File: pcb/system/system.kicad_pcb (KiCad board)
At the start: 2 copper layers, 136.7 x 117.6 mm, 33 parts, among them J1 Raspberry_Pi_4_GPIO, J2 Screw_Terminal_01x02, J3 Servo_1_Header, J4 Servo_2_Header, J5 Screw_Terminal_01x02, J6 Screw_Terminal_01x02, J7 Screw_Terminal_01x02, Q1 BS107A, Q2 BS107A, Q3 BS107A, Q4 BS107A, Q5 IRF520, Q6 IRF520, SW1 SW_SPST, SW2 SW_Push, U1 Teensy4.0

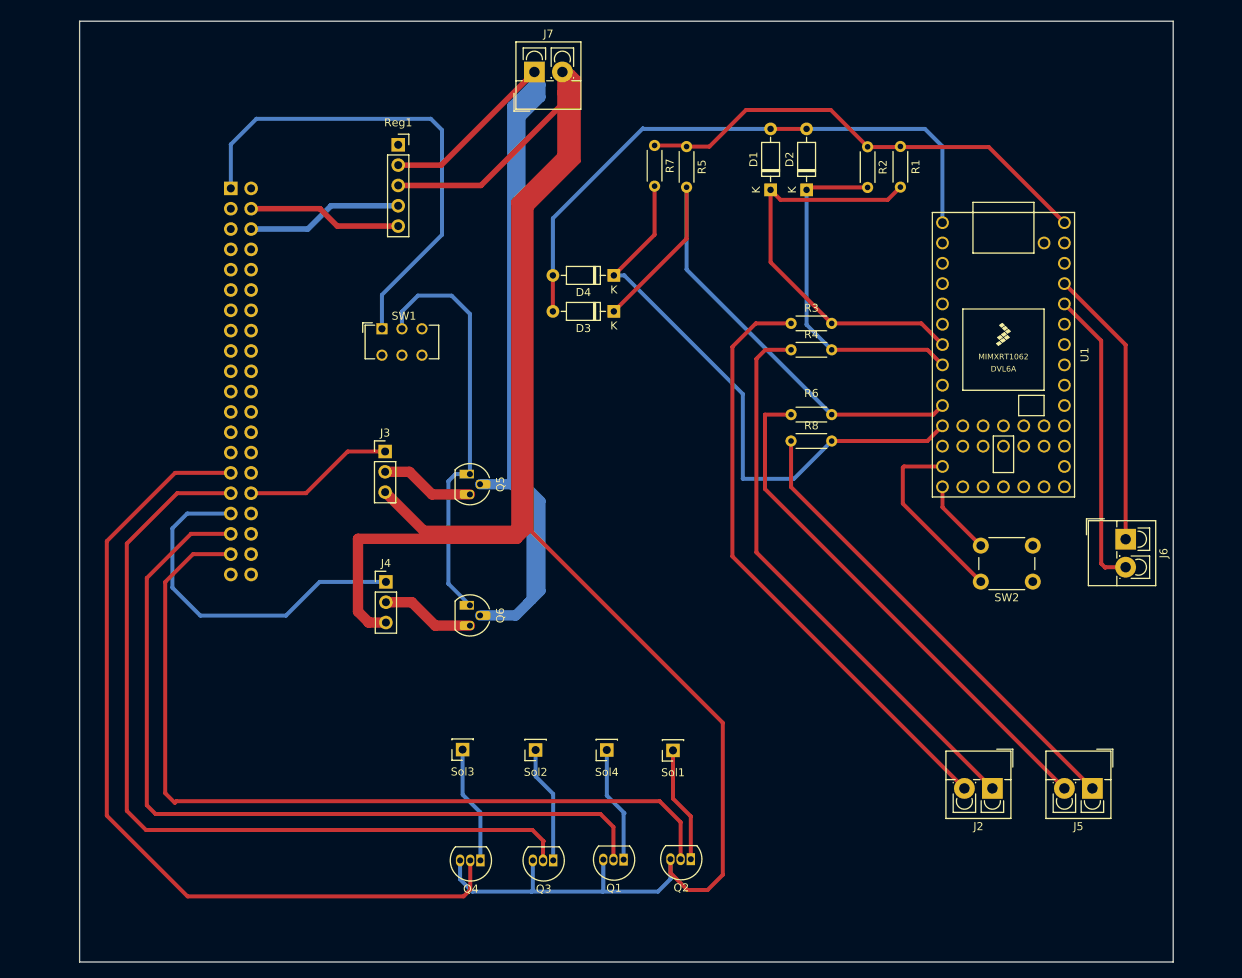
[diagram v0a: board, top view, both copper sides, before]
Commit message: awe
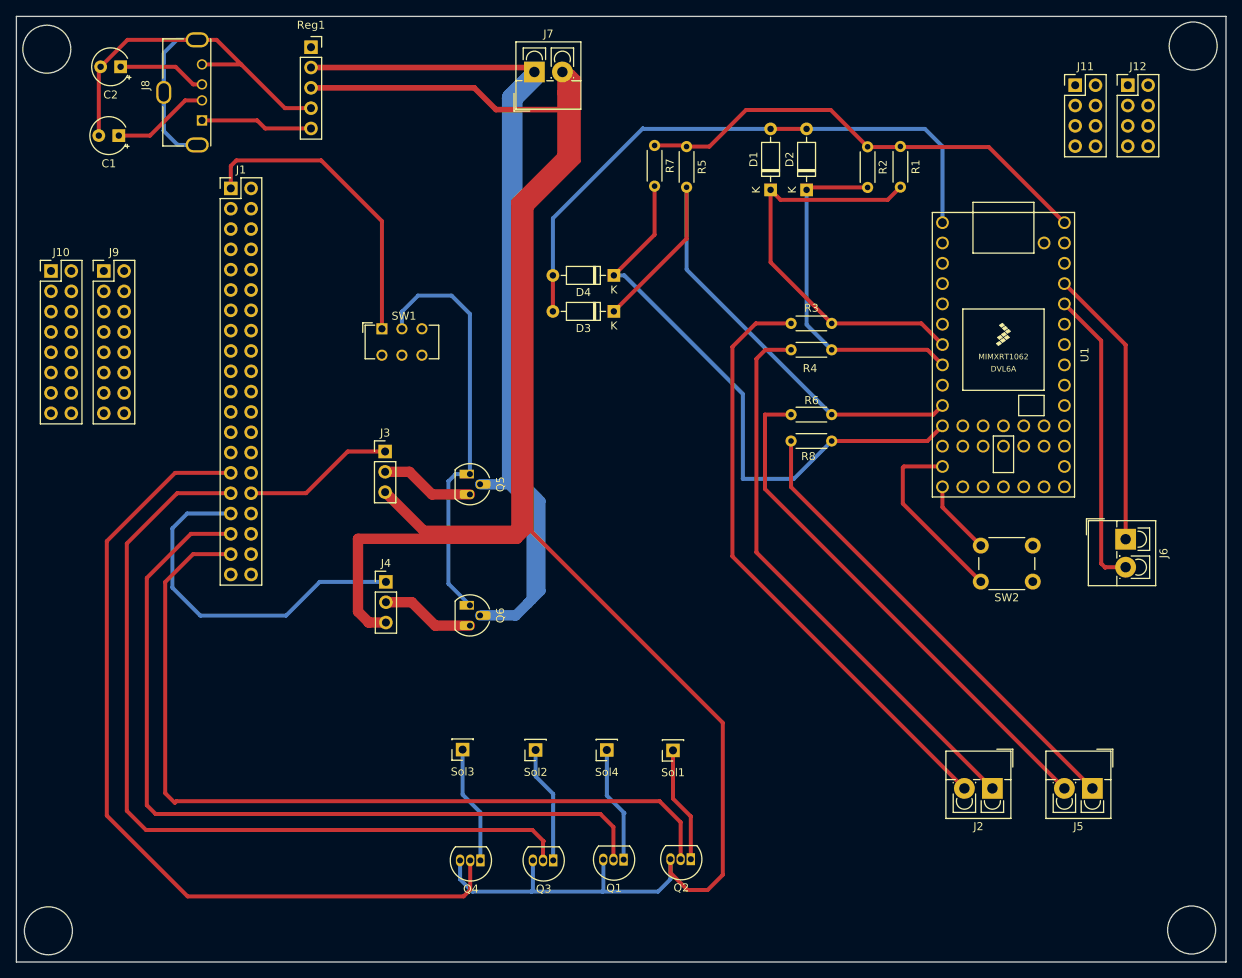
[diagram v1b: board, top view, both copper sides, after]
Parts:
- added C1: 22pF, Capacitor_THT:CP_Radial_Tantal_D4.5mm_P2.50mm, F.Cu at (117.8, 48.6)
- added C2: 22pF, Capacitor_THT:CP_Radial_Tantal_D4.5mm_P2.50mm, F.Cu at (118.0, 40.0)
- added J10: Conn_02x08_Odd_Even, Connector_PinHeader_2.54mm:PinHeader_2x08_P2.54mm_Vertical, F.Cu at (109.3, 65.5)
- added J11: Conn_02x04_Odd_Even, Connector_PinHeader_2.54mm:PinHeader_2x04_P2.54mm_Vertical, F.Cu at (237.3, 42.3)
- added J12: Conn_02x04_Odd_Even, Connector_PinHeader_2.54mm:PinHeader_2x04_P2.54mm_Vertical, F.Cu at (243.9, 42.3)
- added J8: USB_A, Connector_USB:USB_A_Molex_105057_Vertical, F.Cu at (128.2, 46.7)
- added J9: Conn_02x08_Odd_Even, Connector_PinHeader_2.54mm:PinHeader_2x08_P2.54mm_Vertical, F.Cu at (115.9, 65.5)
- J1: footprint Connector_PinSocket_2.54mm:PinSocket_2x20_P2.54mm_Vertical -> Connector_PinHeader_2.54mm:PinHeader_2x20_P2.54mm_Vertical; moved to F.Cu
- R1, R2, R5, R7: value 1.2k -> 1.2kΩ
- R3, R4, R6, R8: value 110 -> 110Ω
- moved Reg1 16.4 mm to (141.8, 37.5)
- turned J1 to 0 degrees
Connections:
- J1 pad 14: GND -> /Ground
- J1 pad 20: GND -> /Ground
- J1 pad 25: GND -> /Ground
- J1 pad 30: GND -> /Ground
- J1 pad 34: GND -> /Ground
- J1 pad 39: GND -> /Ground
- J1 pad 6: GND -> /Ground
- J1 pad 9: GND -> /Ground
- Reg1 pad 5: /5V -> Net-(Reg1-Pad5)
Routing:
- net GND: track 460.6 -> 513.1 mm
- net +8V: track 173.2 -> 127.8 mm
- net /3.3V: track 61.8 -> 38.6 mm
- net /5V: track 19.3 -> 0.00 mm
- net Net-(Reg1-Pad5): track 0.00 -> 14.0 mm
- net Net-(C1-Pad1): track 0.00 -> 12.2 mm
- net Net-(C2-Pad1): track 0.00 -> 11.1 mm
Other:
- board size 136.7 x 117.6 mm -> 151.2 x 118.2 mm
